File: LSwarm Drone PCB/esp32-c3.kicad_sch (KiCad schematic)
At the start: 26 parts, among them U5 ESP32-C3, Y2 40MHz

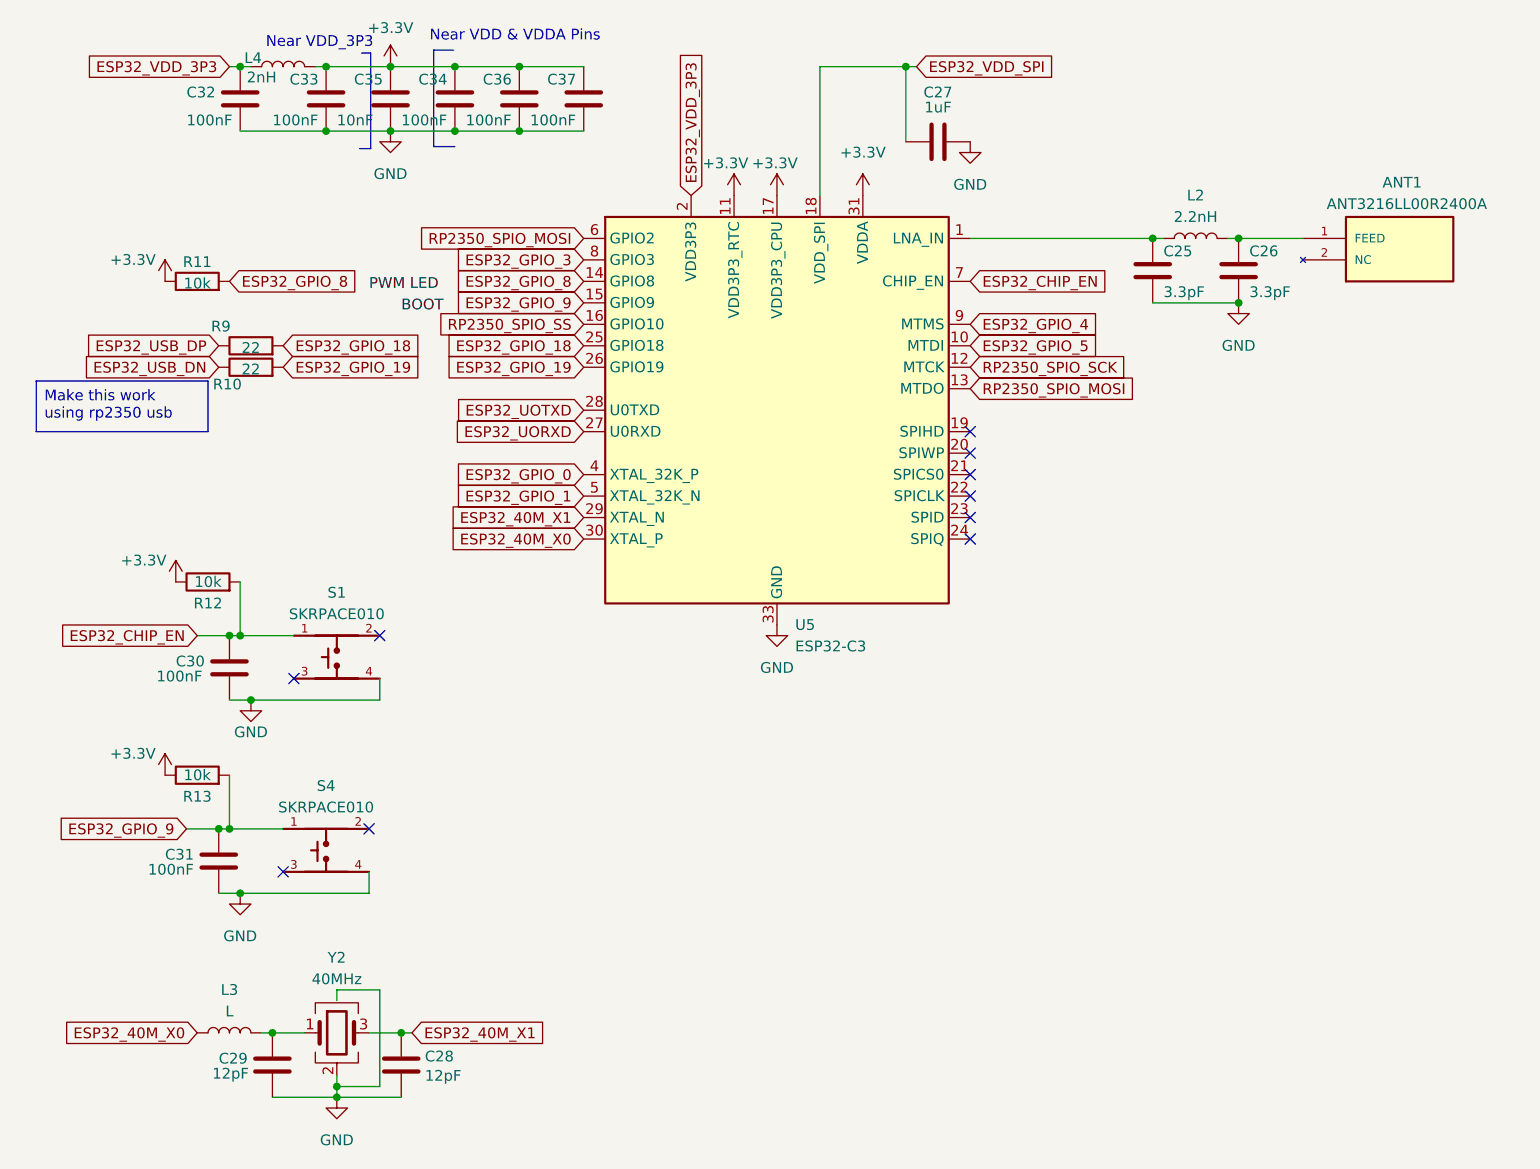
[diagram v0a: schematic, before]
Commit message: sync
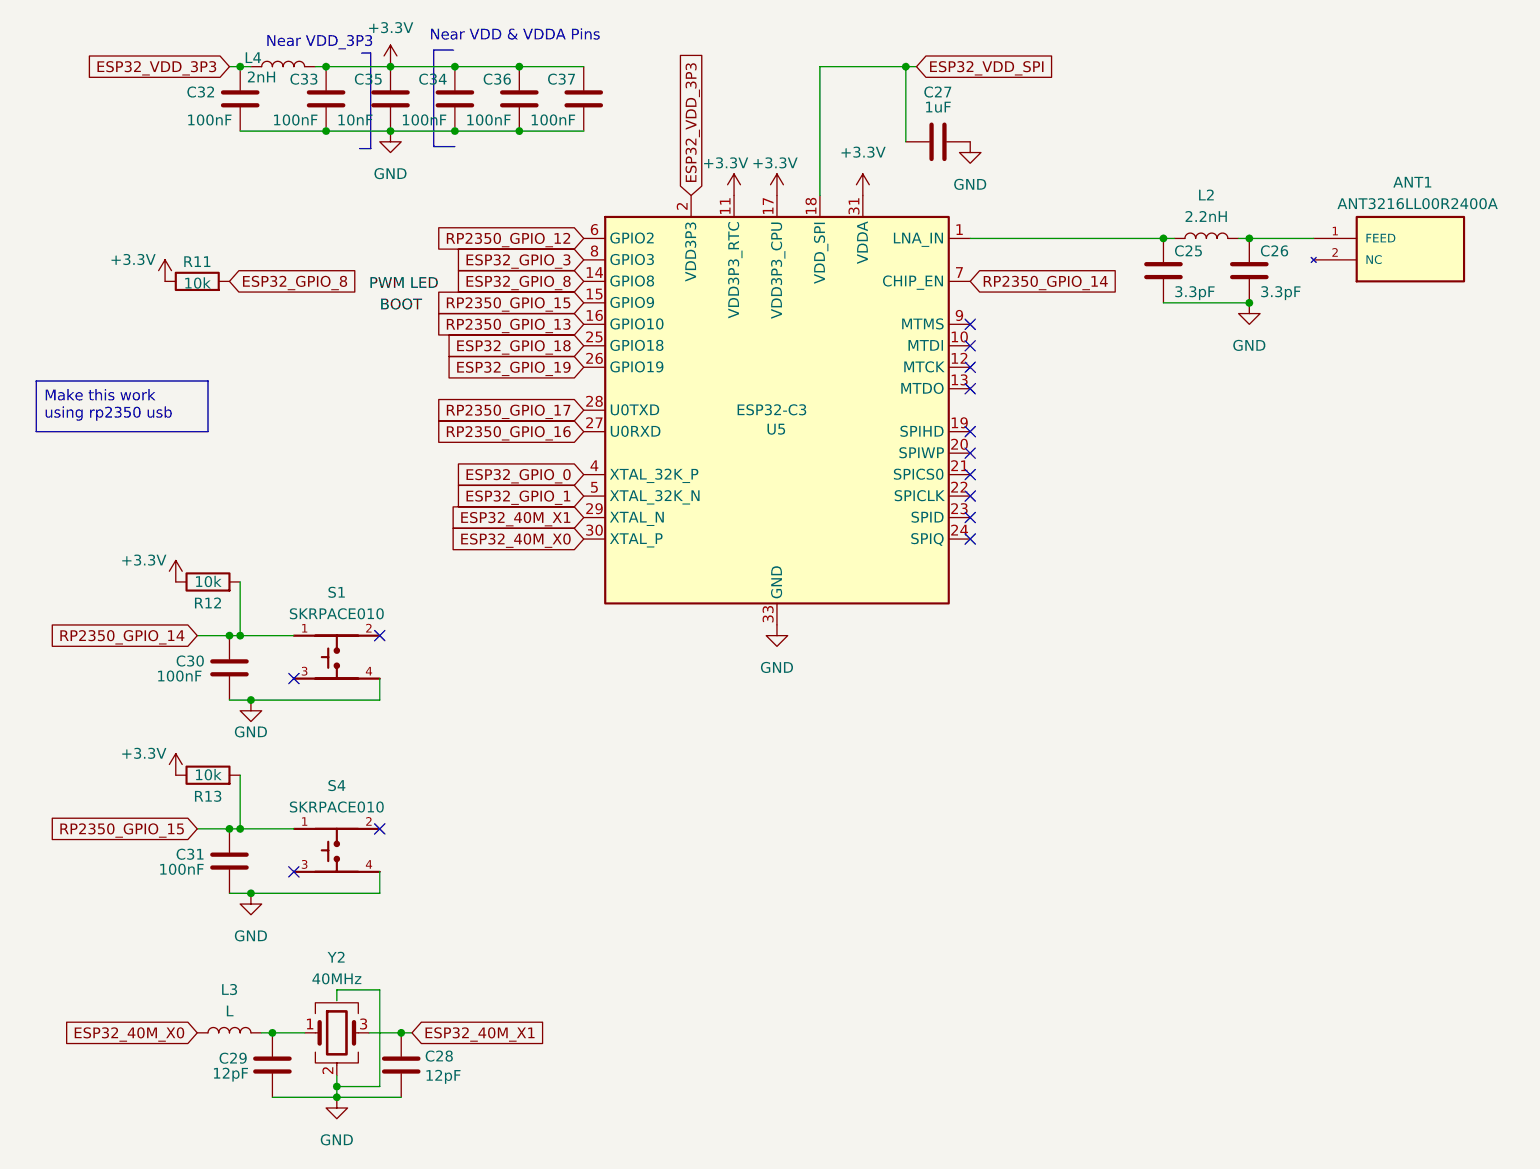
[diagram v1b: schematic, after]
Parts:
- removed R10, R9: 22, symbol Device:R
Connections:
- net ESP32_CHIP_EN renamed RP2350_GPIO_14
- net ESP32_GPIO_4: no longer names the net of U5.9 (MTMS)
- net ESP32_GPIO_5: no longer names the net of U5.10 (MTDI)
- net ESP32_GPIO_9 renamed RP2350_GPIO_15
- net ESP32_UORXD renamed RP2350_GPIO_16
- net ESP32_UOTXD renamed RP2350_GPIO_17
- net RP2350_SPIO_MOSI: no longer names the net of U5.13 (MTDO)
- net RP2350_SPIO_MOSI: no longer U5.6 (GPIO2)
- net RP2350_SPIO_SCK: no longer names the net of U5.12 (MTCK)
- net RP2350_SPIO_SS renamed RP2350_GPIO_13
- new net RP2350_GPIO_12: U5.6 (GPIO2)
- no-connect marks 10 -> 14
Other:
- moved on the sheet: ANT1, C25, C26, C31, L2, R13, S4
